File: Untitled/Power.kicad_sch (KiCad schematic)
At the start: 24 parts, among them J2 USB4125-GF-A-0190, U2 INA180A1, U3 SPX3819M5-L-3-3, U4 SPX3819M5-L-3-3, U5 TPS7A0522PDBZT

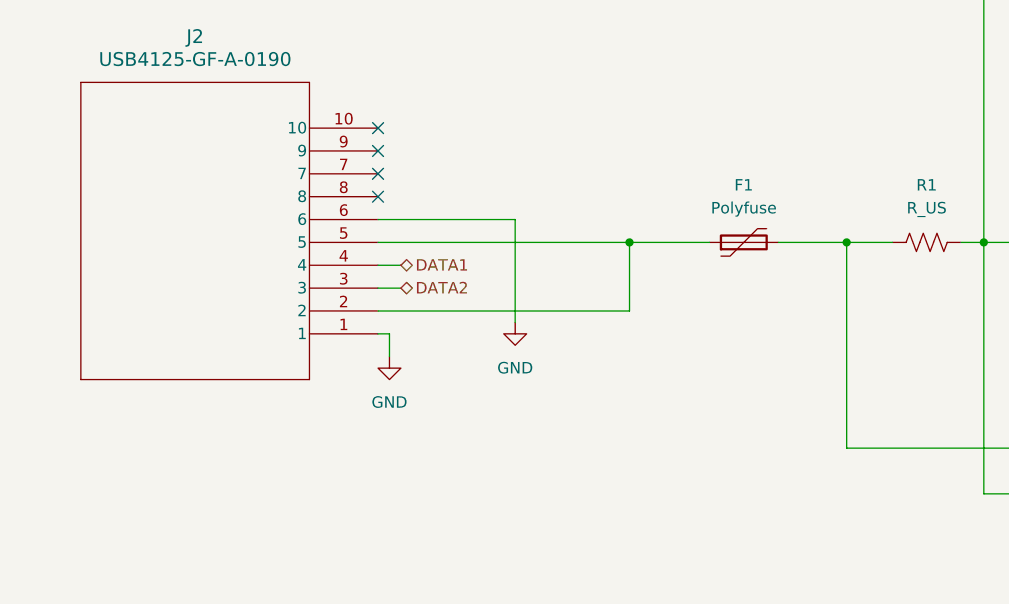
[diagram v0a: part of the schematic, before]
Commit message: revised verison
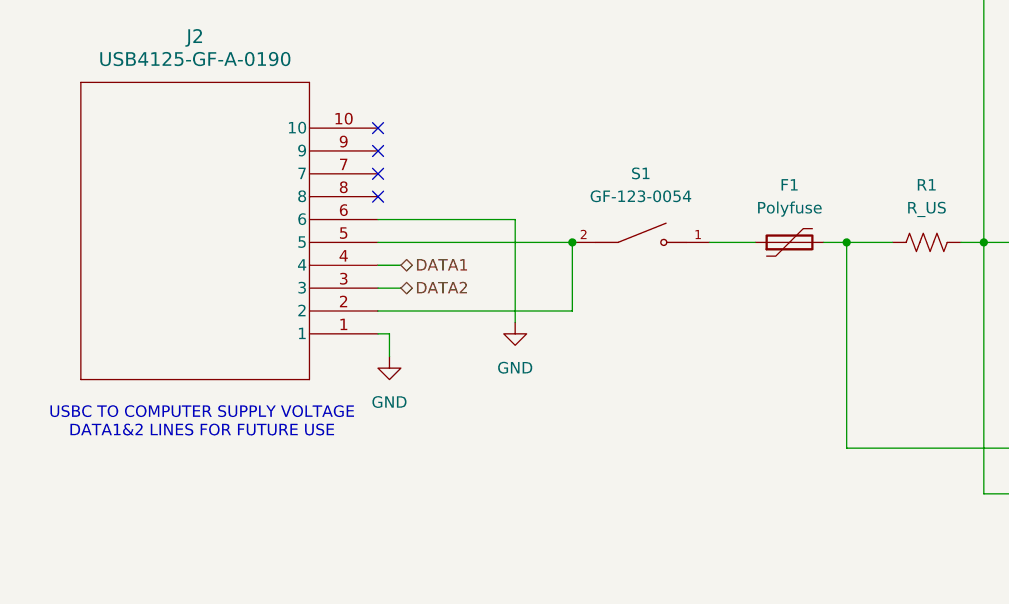
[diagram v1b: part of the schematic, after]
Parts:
- added S1: GF-123-0054, USB-c:SW_GF-123-0054, symbol GF-123-0054:GF-123-0054
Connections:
- net at J2.2, J2.5: now also S1.2; no longer F1.1
- new net: F1.1, S1.1
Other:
- note added: "USBC TO COMPUTER SUPPLY VOLTAGE DATA1&2 LINES FOR FUTURE USE"
- moved on the sheet: F1
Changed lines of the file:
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@@
+		)
+	)
+	(text "USBC TO COMPUTER SUPPLY VOLTAGE\nDATA1&2 LINES FOR FUTURE USE\n"
+		(exclude_from_sim no)
+		(at 37.592 110.236 0)
+		(effects
+			(font
+				(size 1.27 1.27)
+			)
 		)
 	)
@@
 	)
 	(junction
-		(at 85.09 90.17)
-		(diameter 0)
-		(color 0 0 0 0)
-	)
-	(junction
 		(at 207.01 104.14)
 		(diameter 0)
@@
 	)
 	(junction
+		(at 78.74 90.17)
+		(diameter 0)
+		(color 0 0 0 0)
+	)
+	(junction
 		(at 215.9 73.66)
 		(diameter 0)
@@
 	(wire
 		(pts
-			(xy 57.15 90.17) (xy 85.09 90.17)
-		)
-		(stroke
-			(width 0)
-			(type default)
-		)
-	)
-	(wire
-		(pts
 			(xy 207.01 73.66) (xy 215.9 73.66)
 		)
@@
 	(wire
 		(pts
+			(xy 57.15 90.17) (xy 78.74 90.17)
+		)
+		(stroke
+			(width 0)
+			(type default)
+		)
+	)
+	(wire
+		(pts
 			(xy 215.9 106.68) (xy 215.9 104.14)
 		)
@@
 	(wire
 		(pts
-			(xy 57.15 97.79) (xy 85.09 97.79)
-		)
-		(stroke
-			(width 0)
-			(type default)
-		)
-	)
-	(wire
-		(pts
 			(xy 149.86 73.66) (xy 149.86 90.17)
 		)
@@
 	(wire
 		(pts
-			(xy 85.09 90.17) (xy 93.98 90.17)
-		)
-		(stroke
-			(width 0)
-			(type default)
-		)
-	)
-	(wire
-		(pts
 			(xy 250.19 139.7) (xy 250.19 137.16)
 		)
@@
 	(wire
 		(pts
+			(xy 99.06 90.17) (xy 93.98 90.17)
+		)
+		(stroke
+			(width 0)
+			(type default)
+		)
+	)
+	(wire
+		(pts
 			(xy 132.08 118.11) (xy 124.46 118.11)
 		)
@@
 	(wire
 		(pts
-			(xy 85.09 97.79) (xy 85.09 90.17)
-		)
-		(stroke
-			(width 0)
-			(type default)
-		)
-	)
-	(wire
-		(pts
 			(xy 215.9 76.2) (xy 215.9 73.66)
 		)
@@
 	(wire
 		(pts
+			(xy 78.74 97.79) (xy 78.74 90.17)
+		)
+		(stroke
+			(width 0)
+			(type default)
+		)
+	)
+	(wire
+		(pts
 			(xy 247.65 73.66) (xy 256.54 73.66)
 		)
@@
 	(wire
 		(pts
-			(xy 101.6 90.17) (xy 109.22 90.17)
+			(xy 106.68 90.17) (xy 109.22 90.17)
 		)
 		(stroke
@@
 		(pts
 			(xy 109.22 90.17) (xy 114.3 90.17)
+		)
+		(stroke
+			(width 0)
+			(type default)
+		)
+	)
+	(wire
+		(pts
+			(xy 57.15 97.79) (xy 78.74 97.79)
 		)
 		(stroke
@@
 	)
 	(symbol
+		(lib_id "GF-123-0054:GF-123-0054")
+		(at 86.36 90.17 0)
+		(unit 1)
+		(exclude_from_sim no)
+		(in_bom yes)
+		(on_board yes)
+		(dnp no)
+		(fields_autoplaced yes)
+		(property "Reference" "S1"
+			(at 86.36 82.55 0)
+			(effects
+				(font
+					(size 1.27 1.27)
+				)
+			)
+		)
+		(property "Value" "GF-123-0054"
+			(at 86.36 85.09 0)
+			(effects
+				(font
+					(size 1.27 1.27)
+				)
+			)
+		)
+		(property "Footprint" "USB-c:SW_GF-123-0054"
+			(at 86.36 90.17 0)
+			(effects
+				(font
+					(size 1.27 1.27)
+				)
+				(justify bottom)
+				(hide yes)
+			)
+		)
+		(property "Datasheet" ""
+			(at 86.36 90.17 0)
+			(effects
+				(font
+					(size 1.27 1.27)
+				)
+				(hide yes)
+			)
+		)
+		(property "Description" ""
+			(at 86.36 90.17 0)
+			(effects
+				(font
+					(size 1.27 1.27)
+				)
+				(hide yes)
+			)
+		)
+		(property "PARTREV" "May 20, 2003"
+			(at 86.36 90.17 0)
+			(effects
+				(font
+					(size 1.27 1.27)
+				)
+				(justify bottom)
+				(hide yes)
+			)
+		)
+		(property "MANUFACTURER" "CW Industries"
+			(at 86.36 90.17 0)
+			(effects
+				(font
+					(size 1.27 1.27)
+				)
+				(justify bottom)
+				(hide yes)
+			)
+		)
+		(property "MAXIMUM_PACKAGE_HIEGHT" "14.96 mm"
+			(at 86.36 90.17 0)
+			(effects
+				(font
+					(size 1.27 1.27)
+				)
+				(justify bottom)
+				(hide yes)
+			)
+		)
+		(property "STANDARD" "Manufacturer Recommendations"
+			(at 86.36 90.17 0)
+			(effects
+				(font
+					(size 1.27 1.27)
+				)
+				(justify bottom)
+				(hide yes)
+			)
+		)
+		(pin "1"
+		)
+		(pin "2"
+		)
+		(instances
+			(project "Untitled"
+				(path "/ad09c7d2-efab-4012-a18d-674ee0550e5f/5add023e-845f-4db9-9c1a-1a48f6c8ba55"
+					(reference "S1")
+					(unit 1)
+				)
+			)
+		)
+	)
+	(symbol
 		(lib_id "power:GND")
 		(at 137.16 127 0)
@@
 	(symbol
 		(lib_id "Device:Polyfuse")
-		(at 97.79 90.17 90)
+		(at 102.87 90.17 90)
 		(unit 1)
 		(exclude_from_sim no)
@@
 		(fields_autoplaced yes)
 		(property "Reference" "F1"
-			(at 97.79 83.82 90)
+			(at 102.87 83.82 90)
 			(effects
 				(font
@@
 		)
 		(property "Value" "Polyfuse"
-			(at 97.79 86.36 90)
+			(at 102.87 86.36 90)
 			(effects
 				(font
@@
 		)
 		(property "Footprint" "Capacitor_SMD:C_0805_2012Metric_Pad1.18x1.45mm_HandSolder"
-			(at 102.87 88.9 0)
+			(at 107.95 88.9 0)
 			(effects
 				(font
@@
 		)
 		(property "Datasheet" "~"
-			(at 97.79 90.17 0)
+			(at 102.87 90.17 0)
 			(effects
 				(font
@@
 		)
 		(property "Description" "Resettable fuse, polymeric positive temperature coefficient"
-			(at 97.79 90.17 0)
-			(effects
-				(font
+			(at 102.87 90.17 0)
+			(effects
+				(font
